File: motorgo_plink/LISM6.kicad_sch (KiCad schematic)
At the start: 3 parts, among them J23 Conn_01x09_Pin, U10 LSM6DS3TR, U6 LIS3MDLTR

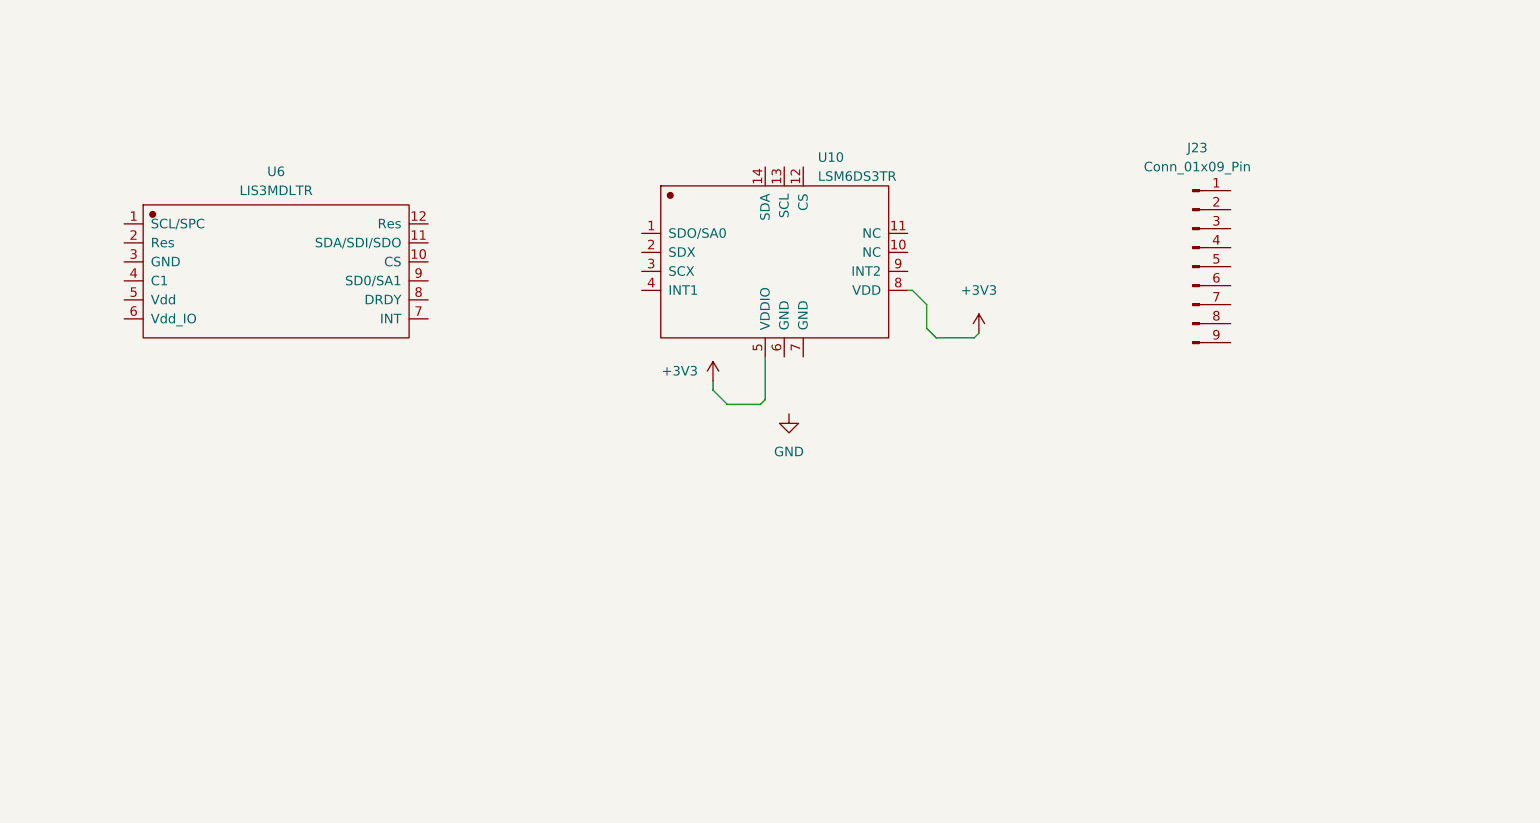
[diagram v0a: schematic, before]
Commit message: WIP update, schematic mainly complete
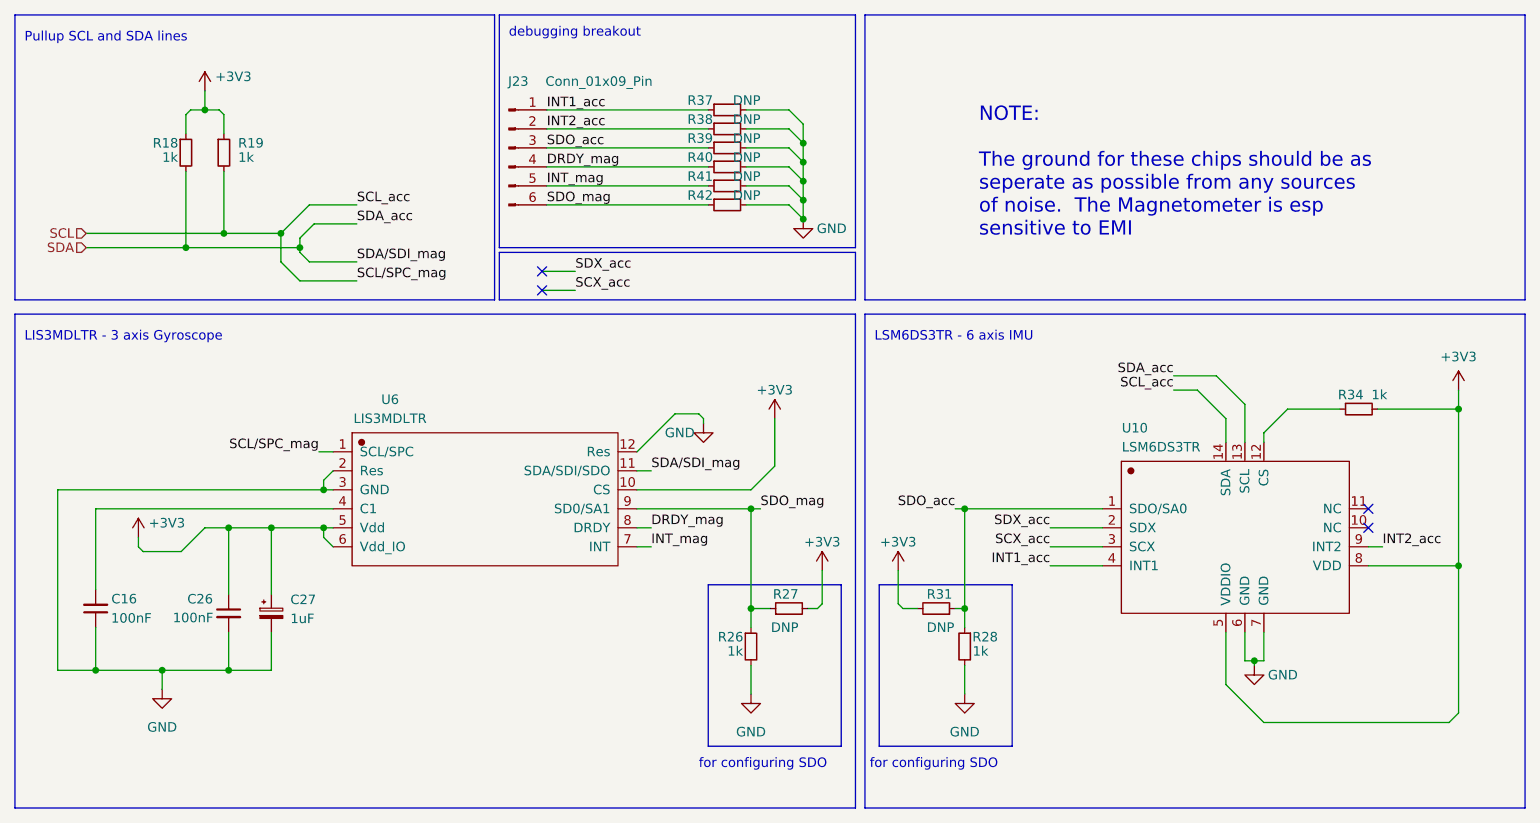
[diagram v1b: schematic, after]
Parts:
- added C16, C26: 100nF, symbol Device:C_Small
- added C27: 1uF, symbol Device:C_Polarized_Small
- added R18, R19, R26, R28, R34: 1k, symbol Device:R_Small
- added R27, R31, R37, R38, R39, R40, R41, R42: DNP, symbol Device:R_Small
- J23: symbol Connector:Conn_01x09_Pin -> Connector:Conn_01x06_Pin
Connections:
- net +3V3: now also U6.10 (CS), U6.5 (Vdd), U6.6 (Vdd_IO), C26.1, C27.1, R18.1, R19.1, R27.2, R31.2, R34.2
- net GND: now also U10.6 (GND), U10.7 (GND), U6.12 (Res), U6.2 (Res), U6.3 (GND), C16.1, C26.2, C27.2, R26.2, R28.2, R37.2, R38.2, R39.2, R40.2, R41.2, R42.2
- net INT1_acc: now reaches J23.1 (Pin_1)
- net INT1_acc: now also U10.4 (INT1), R37.1
- net INT2_acc: now reaches J23.2 (Pin_2)
- net INT2_acc: now also U10.9 (INT2), R38.1
- net SDO_acc: now reaches J23.3 (Pin_3)
- net SDO_acc: now also U10.1 (SDO/SA0), R28.1, R31.1, R39.1
- net DRDY_mag: now reaches J23.4 (Pin_4)
- net DRDY_mag: now also U6.8 (DRDY), R40.1
- net INT_mag: now reaches J23.5 (Pin_5)
- net INT_mag: now also U6.7 (INT), R41.1
- net SDO_mag: now reaches J23.6 (Pin_6)
- net SDO_mag: now also U6.9 (SD0/SA1), R26.1, R27.1, R42.1
- net SCL: now reaches U6.1 (SCL/SPC)
- net SCL: now also U10.14 (SDA), R19.2
- net SDA: now reaches U6.11 (SDA/SDI/SDO)
- net SDA: now also U10.13 (SCL), R18.2
- net at U6.4 (C1): now also C16.2
- net at U10.12 (CS): now also R34.1
- net SDX_acc: now reaches U10.2 (SDX)
- net SCX_acc: now reaches U10.3 (SCX)
- no-connect marks 0 -> 4
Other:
- note added: "LIS3MDLTR - 3 axis Gyroscope"
- note added: "LSM6DS3TR - 6 axis IMU"
- note added: "NOTE: The ground for these chips should be as seperate as possible from any sources of noise. The Magnetometer is esp sensitive to EMI"
- note added: "Pullup SCL and SDA lines"
- note added: "debugging breakout"
- note added: "for configuring SDO"
- moved on the sheet: U10, U6
